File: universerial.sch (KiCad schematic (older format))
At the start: 11 parts

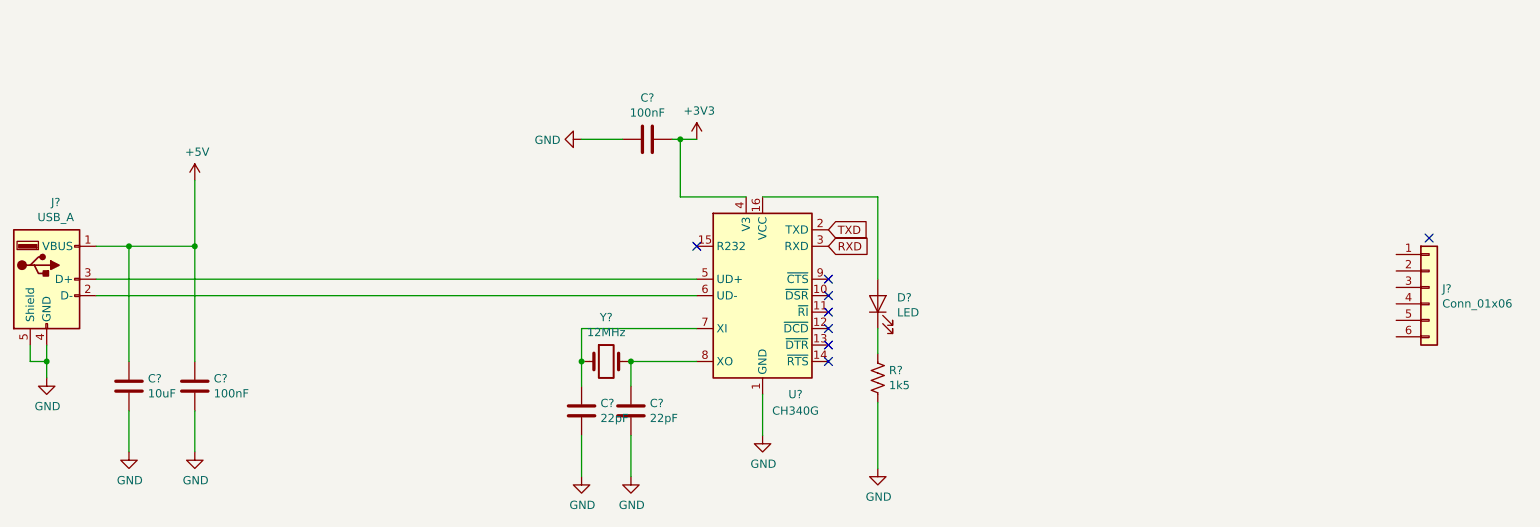
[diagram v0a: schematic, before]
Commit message: Finish schematic.
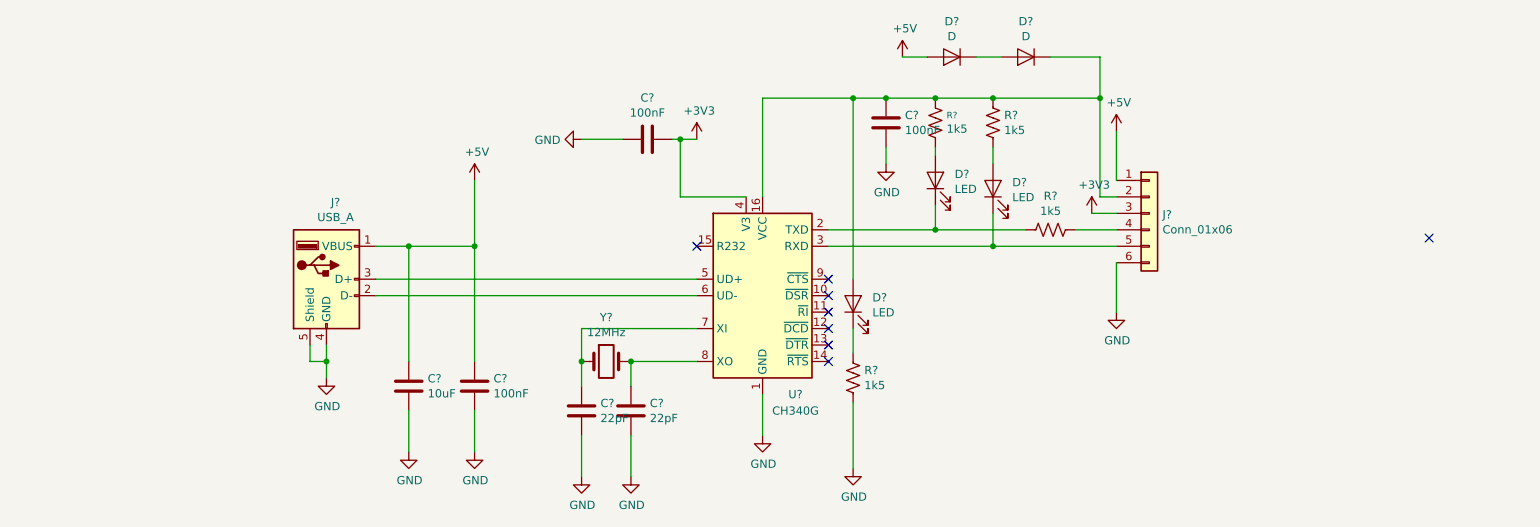
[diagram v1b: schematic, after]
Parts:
- added C?: 100nF, symbol Device:C
- added D? (x2): D, symbol Device:D
- added D? (x2): LED, symbol Device:LED
- added R? (x3): 1k5, symbol Device:R_US
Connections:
- net RXD is gone; now on an unnamed net: U?.3 (RXD)
- net +3V3: now also J?.3 (Pin_3)
- net +5V: now also J?.1 (Pin_1), D?.2 (A)
- net GND: now also J?.6 (Pin_6), C?.2
- net at D?.2 (A), U?.16 (VCC): now also J?.2 (Pin_2), C?.1, D?.1 (K), R?.1, R?.1
- net at J?.4 (Pin_4): now also R?.1
- net at J?.5 (Pin_5): now also D?.1 (K)
- net TXD: no longer names the net of U?.2 (TXD)
- net TXD: now also D?.1 (K), R?.2
- new net: D?.1 (K), D?.2 (A)
- new net: D?.2 (A), R?.2 (x2)
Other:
- moved on the sheet: C?, D?, J?, R?
